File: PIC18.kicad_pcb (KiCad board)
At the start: 4 copper layers, 75.8 x 75.6 mm, 75 parts, among them J1 Conn_02x20_Odd_Even, J10 Port B, J11 Port C, J12 Port D, J13 Conn_01x03, J14 Conn_01x03, J15 Conn_01x03, J16 Conn_01x03, J2 Conn_01x06, J3 USB_A, J4 Conn_01x03, J5 Conn_01x02, J6 Conn_01x02, J7 USB_OTG, J8 Port A, J9 Port E, U1 PIC18F4620, U2 LM4040DBZ-4.1, U3 FT230XS, Y1 8 MHz

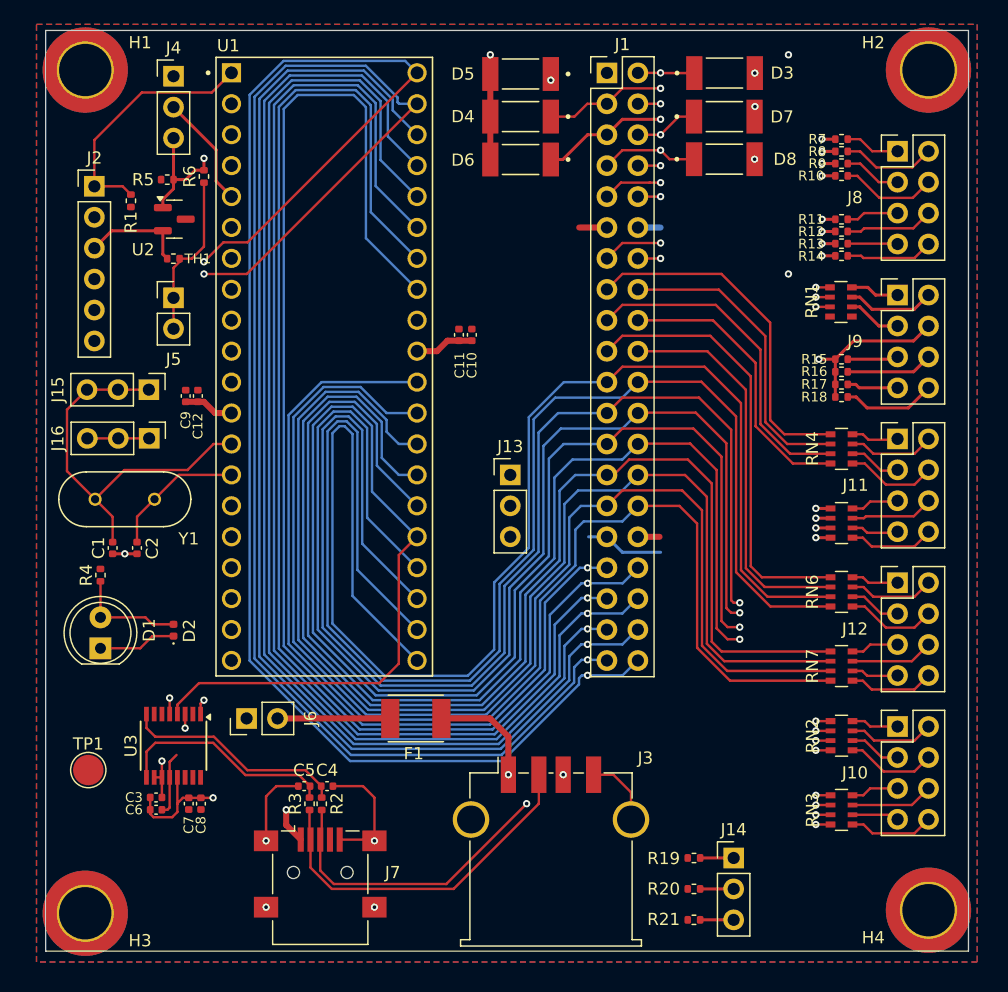
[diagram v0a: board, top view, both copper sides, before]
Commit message: Silkscreen edits
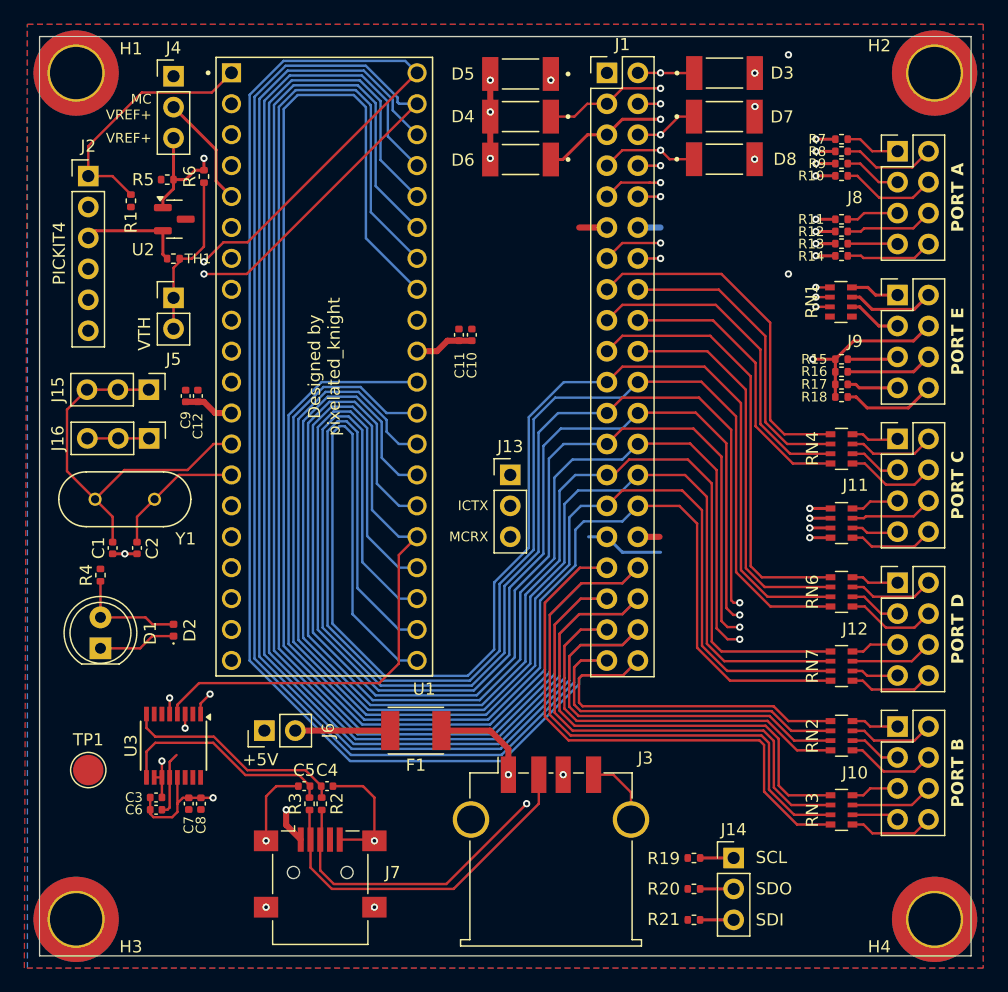
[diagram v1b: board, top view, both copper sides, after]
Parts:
- moved J6 1.77 mm to (117.5, 123.0)
- moved F1 1.00 mm to (129.9, 123.0)
- moved J2 0.98 mm to (103.0, 77.5)
- moved H3 0.90 mm to (102.0, 138.5)
- moved H4 0.90 mm to (172.5, 138.5)
- moved H1 0.79 mm to (102.0, 69.0)
- moved H2 0.56 mm to (172.5, 69.0)
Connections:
- net /ICTX renamed /TXD
- J13 pad 3: /RC6/TX/CK -> /RC7/RX/DT
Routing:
- net /RC7/RX/DT: track 114.1 -> 124.0 mm
- net /RC6/TX/CK: track 155.3 -> 148.7 mm
- net /RB3/AN9/CCP2(1): track 140.7 -> 146.2 mm, vias 2 -> 0
- net /RB1/INT1/AN10: track 148.0 -> 153.5 mm, vias 2 -> 0
- net /RB7/KBI3/PGD: track 158.4 -> 163.2 mm, vias 3 -> 1
- net /RB5/KBI1/PGM: track 130.5 -> 135.1 mm, vias 2 -> 0
- net /RB0/INT0/FLT0/AN12: track 148.9 -> 151.2 mm, vias 2 -> 0
- net /RB2/INT2/AN8: track 141.4 -> 143.7 mm, vias 2 -> 0
- net /RB6/KBI2/PGC: track 158.1 -> 159.8 mm, vias 3 -> 1
- net /RB4/KBI0/AN11: track 131.2 -> 132.7 mm, vias 2 -> 0
- net VCC: track 18.6 -> 17.1 mm
- net GND: track 76.9 -> 75.5 mm, vias 11 -> 13
- net Net-(J3-VBUS): track 32.7 -> 31.7 mm
- net /RD2/PSP2: track 117.2 -> 118.0 mm
- net /RD3/PSP3: track 115.4 -> 116.2 mm
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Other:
- board size 75.8 x 75.6 mm -> 76.5 x 75.5 mm
- board text added: "+5V"
- board text added: "Designed by pixelated_knight"
- board text added: "ICTX"
- board text added: "MC VREF+"
- board text added: "MCRX"
- board text added: "PICKIT4"
- board text added: "PORT A"
- board text added: "PORT B"
- board text added: "PORT C"
- board text added: "PORT D"
- board text added: "PORT E"
- board text added: "SCL"
- board text added: "SDI"
- board text added: "SDO"
- board text added: "VREF+"
- board text added: "VTH"

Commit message: JLCPCB parody edits
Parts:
- C10, C12: value .1uf -> 100nf
